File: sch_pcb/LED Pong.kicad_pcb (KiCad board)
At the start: 2 copper layers, 69.6 x 54.4 mm, 14 parts, among them SW1 SW_Push, SW2 SW_Push

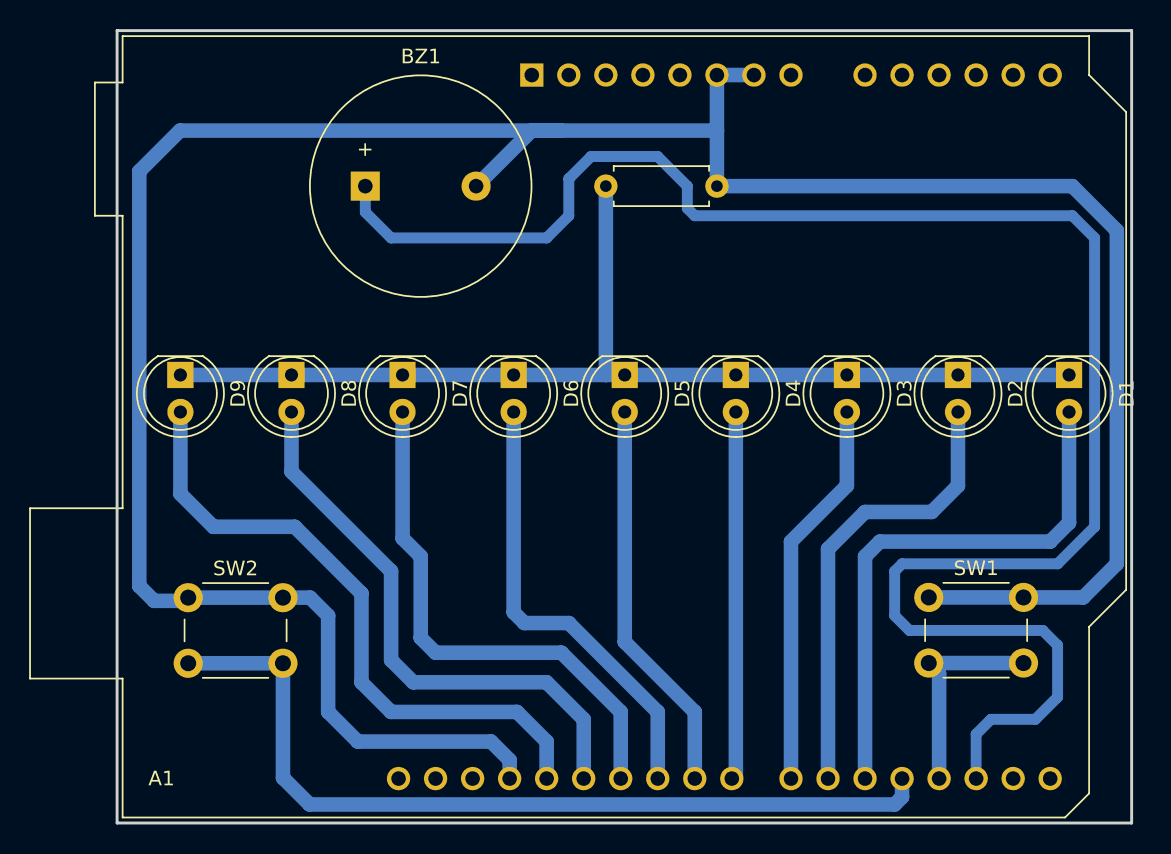
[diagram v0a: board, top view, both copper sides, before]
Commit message: update brd
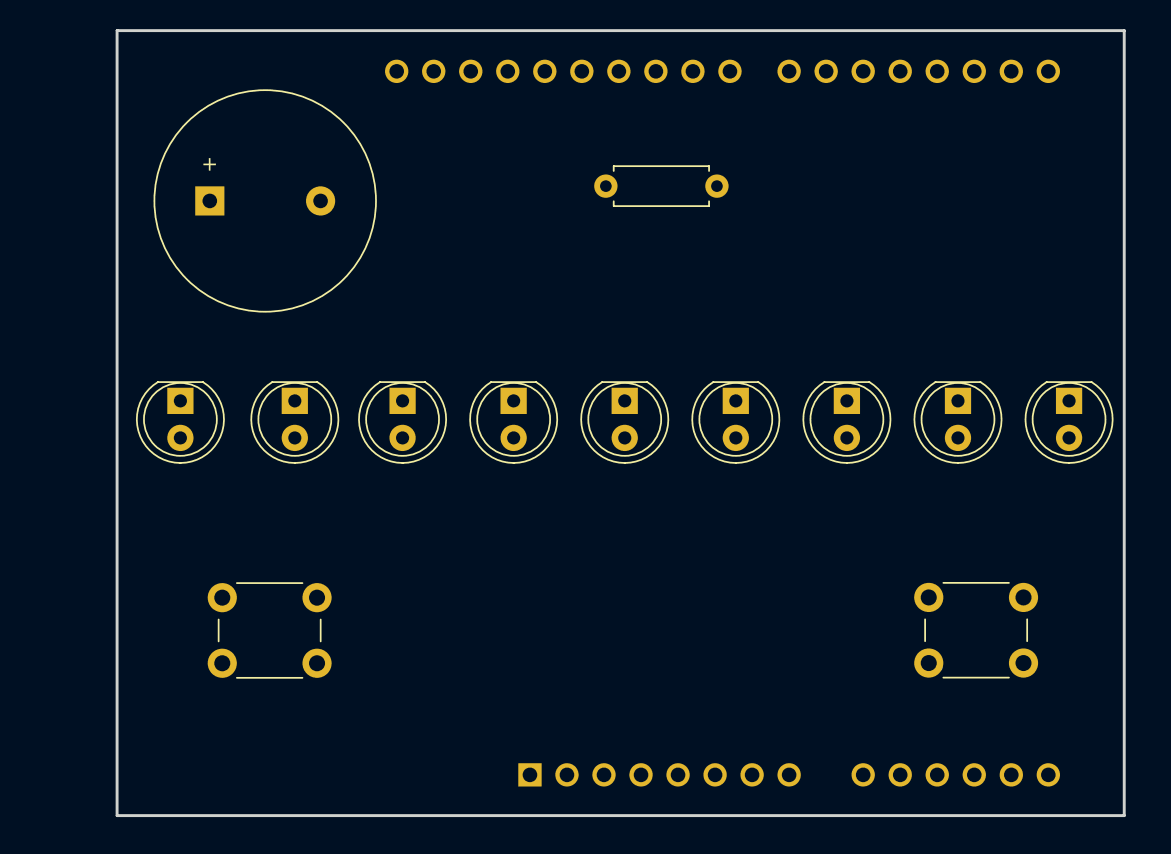
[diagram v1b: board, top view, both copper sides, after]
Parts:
- A1: moved to B.Cu
- moved A1 48.0 mm to (132.0, 119.1)
- moved BZ1 10.7 mm to (110.0, 79.8)
- moved SW2 2.34 mm to (110.8, 107.0)
- moved D8 1.79 mm to (115.8, 93.5)
- moved D1 1.78 mm to (168.9, 93.5)
- moved D2 1.78 mm to (161.3, 93.5)
- moved D3 1.78 mm to (153.7, 93.5)
- moved D4 1.78 mm to (146.1, 93.5)
- moved D5 1.78 mm to (138.5, 93.5)
- moved D6 1.78 mm to (130.8, 93.5)
- moved D7 1.78 mm to (123.2, 93.5)
- moved D9 1.78 mm to (108.0, 93.5)
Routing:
- net GND: track 187.9 -> 0.00 mm
- net Net-(A1-D2): track 122.7 -> 0.00 mm
- net Net-(D1-K): track 73.9 -> 0.00 mm
- net Net-(A1-D4): track 59.1 -> 0.00 mm
- net /D13: track 43.9 -> 0.00 mm
- net /D12: track 38.8 -> 0.00 mm
- net /D5: track 37.8 -> 0.00 mm
- net /D11: track 36.4 -> 0.00 mm
- net /D6: track 31.5 -> 0.00 mm
- net /D10: track 31.0 -> 0.00 mm
- net /D9: track 27.1 -> 0.00 mm
- net /D7: track 26.7 -> 0.00 mm
- net /D8: track 25.3 -> 0.00 mm
- net Net-(A1-D3): track 15.6 -> 0.84 mm
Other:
- board size 69.6 x 54.4 mm -> 69.1 x 53.8 mm
